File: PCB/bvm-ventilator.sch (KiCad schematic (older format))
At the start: 1 part, among them U13 IEC_CONNECTOR

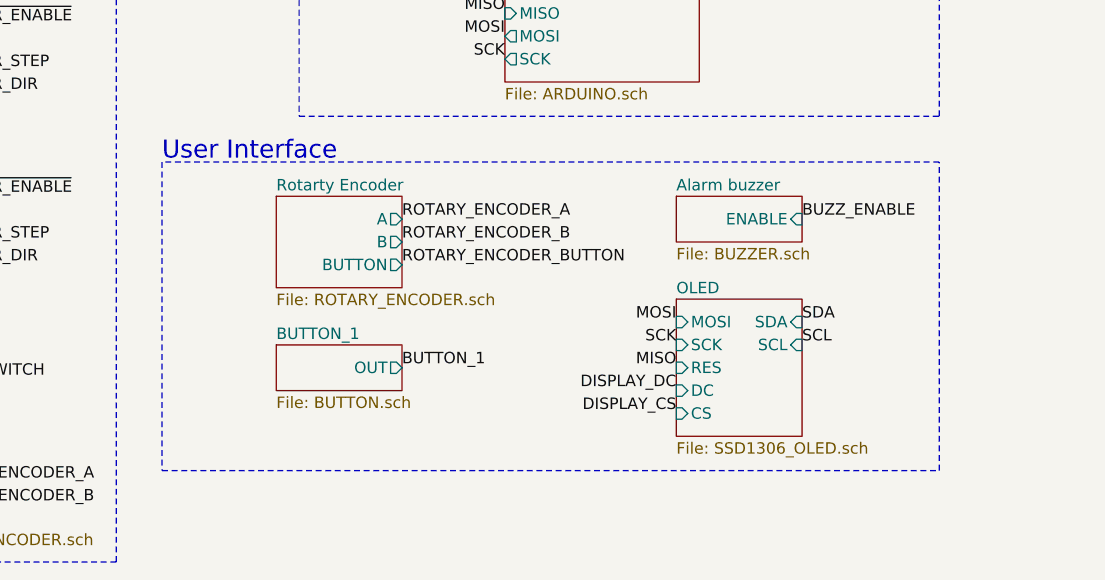
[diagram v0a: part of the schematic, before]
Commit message: Checkpoint
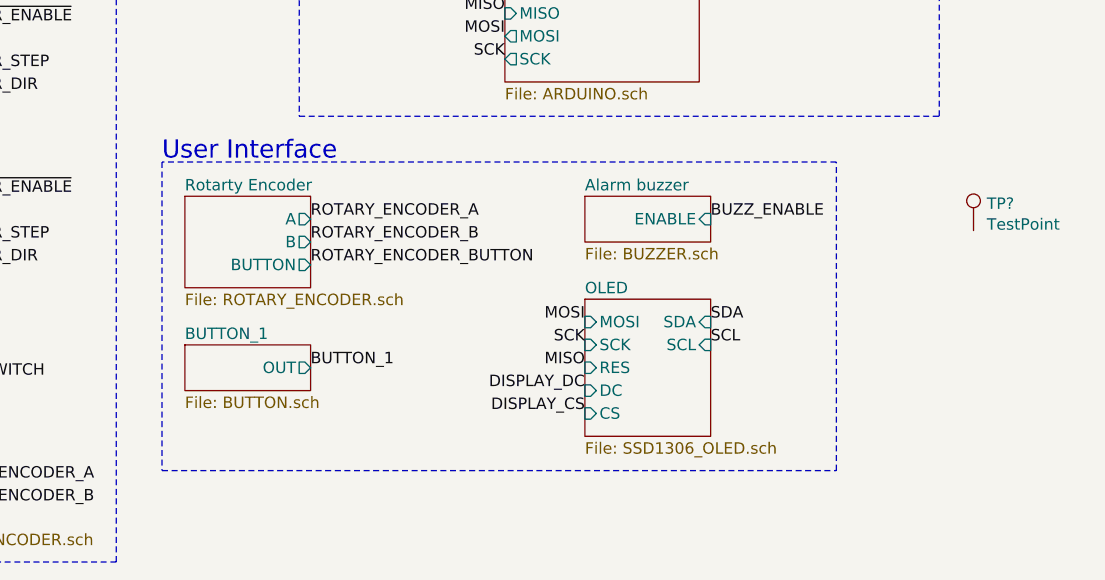
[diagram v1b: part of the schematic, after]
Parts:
- added TP?: TestPoint, symbol Connector:TestPoint
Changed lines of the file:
@@
 $EndSheet
 $Sheet
-S 7200 4850 550  200
+S 6800 4850 550  200
 U 5E8EB699
 F0 "Alarm buzzer" 50
 F1 "BUZZER.sch" 50
-F2 "ENABLE" I R 7750 4950 50
-$EndSheet
-$Sheet
-S 7200 5300 550  600
+F2 "ENABLE" I R 7350 4950 50
+$EndSheet
+$Sheet
+S 6800 5300 550  600
 U 5E8F3A13
 F0 "OLED" 50
 F1 "SSD1306_OLED.sch" 50
-F2 "SCL" I R 7750 5500 50
-F3 "SDA" I R 7750 5400 50
-F4 "MOSI" I L 7200 5400 50
-F5 "SCK" I L 7200 5500 50
-F6 "DC" I L 7200 5700 50
-F7 "CS" I L 7200 5800 50
-F8 "RES" I L 7200 5600 50
+F2 "SCL" I R 7350 5500 50
+F3 "SDA" I R 7350 5400 50
+F4 "MOSI" I L 6800 5400 50
+F5 "SCK" I L 6800 5500 50
+F6 "DC" I L 6800 5700 50
+F7 "CS" I L 6800 5800 50
+F8 "RES" I L 6800 5600 50
 $EndSheet
 $Sheet
@@
 Text Label 6450 3900 2    50   ~ 0
 SCL
-Text Label 7750 5400 0    50   ~ 0
-SDA
-Text Label 7750 5500 0    50   ~ 0
+Text Label 7350 5400 0    50   ~ 0
+SDA
+Text Label 7350 5500 0    50   ~ 0
 SCL
 Text Label 3400 2800 0    50   ~ 0
@@
 Text Label 7300 3950 0    50   ~ 0
 STEPPER_DIR
-Text Label 7750 4950 0    50   ~ 0
+Text Label 7350 4950 0    50   ~ 0
 BUZZ_ENABLE
 Text Label 6450 3150 2    50   ~ 0
@@
 VBATT_SENSE
 $Sheet
-S 5450 4850 550  400
+S 5050 4850 550  400
 U 5E8BEE14
 F0 "Rotarty Encoder" 50
 F1 "ROTARY_ENCODER.sch" 50
-F2 "A" O R 6000 4950 50
-F3 "B" O R 6000 5050 50
-F4 "BUTTON" O R 6000 5150 50
-$EndSheet
-Text Label 6000 4950 0    50   ~ 0
+F2 "A" O R 5600 4950 50
+F3 "B" O R 5600 5050 50
+F4 "BUTTON" O R 5600 5150 50
+$EndSheet
+Text Label 5600 4950 0    50   ~ 0
 ROTARY_ENCODER_A
-Text Label 6000 5050 0    50   ~ 0
+Text Label 5600 5050 0    50   ~ 0
 ROTARY_ENCODER_B
-Text Label 6000 5150 0    50   ~ 0
+Text Label 5600 5150 0    50   ~ 0
 ROTARY_ENCODER_BUTTON
 Text Label 7300 3350 0    50   ~ 0
@@
 ROTARY_ENCODER_BUTTON
 $Sheet
-S 5450 5500 550  200
+S 5050 5500 550  200
 U 5E8CBD7F
 F0 "BUTTON_1" 50
 F1 "BUTTON.sch" 50
-F2 "OUT" O R 6000 5600 50
-$EndSheet
-Text Label 6000 5600 0    50   ~ 0
+F2 "OUT" O R 5600 5600 50
+$EndSheet
+Text Label 5600 5600 0    50   ~ 0
 BUTTON_1
 Text Label 6450 3450 2    50   ~ 0
@@
 Text Label 6450 3550 2    50   ~ 0
 DISPLAY_DC
-Text Label 7200 5700 2    50   ~ 0
+Text Label 6800 5700 2    50   ~ 0
 DISPLAY_DC
-Text Label 7200 5800 2    50   ~ 0
+Text Label 6800 5800 2    50   ~ 0
 DISPLAY_CS
-Text Label 7200 5600 2    50   ~ 0
+Text Label 6800 5600 2    50   ~ 0
 MISO
-Text Label 7200 5400 2    50   ~ 0
+Text Label 6800 5400 2    50   ~ 0
 MOSI
-Text Label 7200 5500 2    50   ~ 0
+Text Label 6800 5500 2    50   ~ 0
 SCK
 Wire Notes Line
 	4950 4700 4950 6050
 Wire Notes Line
-	4950 6050 8350 6050
-Wire Notes Line
-	8350 6050 8350 4700
-Wire Notes Line
-	8350 4700 4950 4700
+	4950 6050 7900 6050
+Wire Notes Line
+	7900 6050 7900 4700
+Wire Notes Line
+	7900 4700 4950 4700
 Text Notes 2750 3850 0    79   ~ 0
 Motion Control
@@
 Text Notes 4550 2950 0    79   ~ 0
 Misc.
+$Comp
+L Connector:TestPoint TP?
+U 1 1 5E8ED4B0
+P 8500 5000
+F 0 "TP?" H 8558 5118 50  0000 L CNN
+F 1 "TestPoint" H 8558 5027 50  0000 L CNN
+F 2 "" H 8700 5000 50  0001 C CNN
+F 3 "~" H 8700 5000 50  0001 C CNN
+	1    8500 5000
+	1    0    0    -1
+$EndComp
 $EndSCHEMATC
